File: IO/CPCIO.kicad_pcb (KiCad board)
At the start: 2 copper layers, 99.1 x 52.9 mm, 57 parts, among them IC107 8255A, IC301 LM358, J1 Tape in, J2 Tape out, J3 Motor, J901 Conn_01x07_Male, J902 Conn_01x08_Male, Q101 BC337, Q901 BC337, U1 74LS688

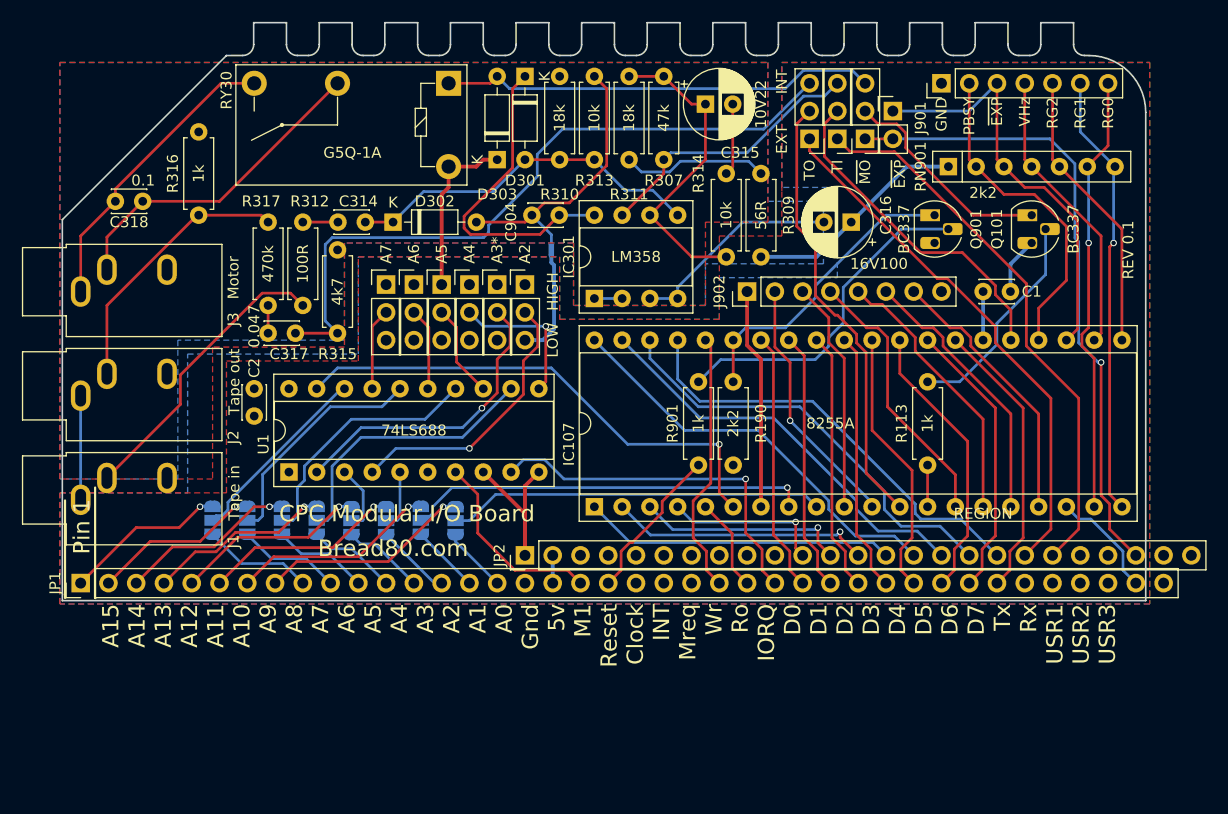
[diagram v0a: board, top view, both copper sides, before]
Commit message: Long overdue update...
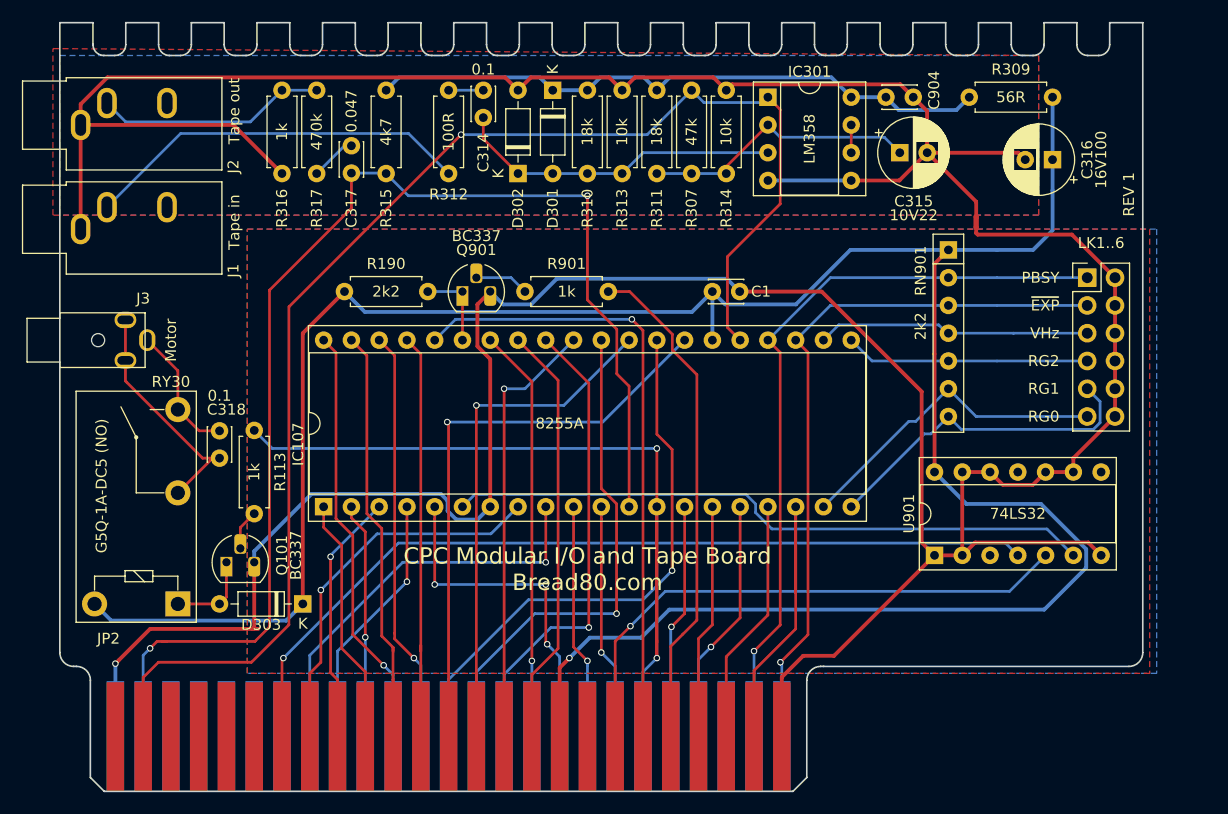
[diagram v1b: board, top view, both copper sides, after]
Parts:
- removed C2: 0.1nF, Capacitor_THT:C_Disc_D3.0mm_W2.0mm_P2.50mm
- removed J901: Conn_01x07_Male, Connector_PinHeader_2.54mm:PinHeader_1x07_P2.54mm_Vertical
- removed J902: Conn_01x08_Male, Connector_PinHeader_2.54mm:PinHeader_1x08_P2.54mm_Vertical
- removed JP10: A14A6, Connector_PinHeader_2.54mm:PinHeader_1x03_P2.54mm_Vertical
- removed JP11, JP17, JP18, JP19: A10A2, Connector_PinHeader_2.54mm:PinHeader_1x03_P2.54mm_Vertical
- removed JP12: A15A7, Connector_PinHeader_2.54mm:PinHeader_1x03_P2.54mm_Vertical
- removed JP13, JP14, JP15, JP16, JP3, JP4, JP7, JP8: Jumper_3_Bridged12, Jumper:SolderJumper-3_P1.3mm_Open_RoundedPad1.0x1.5mm
- removed JP5: A12A4, Connector_PinHeader_2.54mm:PinHeader_1x03_P2.54mm_Vertical
- removed JP6: A13A5, Connector_PinHeader_2.54mm:PinHeader_1x03_P2.54mm_Vertical
- removed JP9: A11A3, Connector_PinHeader_2.54mm:PinHeader_1x03_P2.54mm_Vertical
- removed LK913: Jumper_NO_Small, Connector_PinHeader_2.54mm:PinHeader_1x02_P2.54mm_Vertical
- removed U1: 74LS688, Package_DIP:DIP-20_W7.62mm_Socket
- added LK1..6: Settings, Connector_PinHeader_2.54mm:PinHeader_2x06_P2.54mm_Vertical, F.Cu at (247.7, 123.8)
- added U901: 74LS32, Package_DIP:DIP-14_W7.62mm_Socket, F.Cu at (233.7, 149.2)
- J3: footprint Connector_Audio:Jack_3.5mm_CUI_SJ1-3533NG_Horizontal -> CPCModular:CUI_MJ1_2503A
- JP1: value RC2014Bus -> CPCM_IOSound_EdgeBottom; footprint Connector_PinHeader_2.54mm:PinHeader_1x40_P2.54mm_Vertical -> CPCModular:Edge25_2.54PS; moved to B.Cu
- JP2: value RC2014ExtendedBus -> CPCM_IOSound_EdgeTop; footprint Connector_PinHeader_2.54mm:PinHeader_1x25_P2.54mm_Vertical -> CPCModular:Edge25_2.54PS
- JP20: moved to F.Cu
- RY30: value G5Q-1A -> G5Q-1A-DC5 (NO)
- moved Q101 80.2 mm to (168.9, 149.9), turned to 0 degrees
- moved R113 61.7 mm to (171.4, 137.8), turned to 270 degrees
- moved RY30 53.7 mm to (164.5, 153.7), turned to 90 degrees
- moved D303 44.4 mm to (175.9, 153.7), turned to 180 degrees
- moved Q901 43.7 mm to (190.5, 125.1), turned to 0 degrees
- moved JP2 41.7 mm to (158.8, 167.6)
- moved JP20 38.9 mm to (237.5, 118.7)
- moved R190 38.9 mm to (179.7, 125.1), turned to 0 degrees
- moved C904 31.8 mm to (229.2, 107.3), turned to 0 degrees
- moved R309 30.4 mm to (244.5, 107.3), turned to 180 degrees
- moved J1 24.8 mm to (155.6, 119.4)
- moved J2 24.8 mm to (155.6, 109.9)
- moved C1 24.8 mm to (213.4, 125.1)
- moved IC107 24.8 mm to (177.8, 144.8)
- moved IC301 24.3 mm to (218.4, 107.3), turned to 0 degrees
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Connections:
- C317 pad 2: /IO_SOUND/Tape/CASWRINT -> /IO_SOUND/CASWR
- IC107 pad 12: /IO_SOUND/WR_DATA -> /IO_SOUND/CASWR
- IC107 pad 13: Net-(IC107-Pad13) -> /IO_SOUND/MOTOR
- IC107 pad 25: /IO_SOUND/RD_DATA -> /IO_SOUND/CASRD
- IC107 pad 8: /IO_SOUND/A9A1 -> A9
- IC107 pad 9: /IO_SOUND/A8A0 -> A8
- IC301 pad 1: Net-(IC301-Pad1) -> /IO_SOUND/CASRD
- IC301 pad 2: Net-(IC301-Pad1) -> Net-(C315-Pad1)
- IC301 pad 3: GNDA -> Net-(C314-Pad1)
- IC301 pad 5: Net-(C314-Pad1) -> GNDA
- IC301 pad 6: Net-(C315-Pad1) -> Net-(IC301-Pad6)
- IC301 pad 7: /IO_SOUND/Tape/CASRDINT -> Net-(IC301-Pad6)
- J3 pad S: Net-(C318-Pad1) -> Net-(C318-Pad2)
- J3 pad T: Net-(C318-Pad2) -> Net-(C318-Pad1)
- JP1 pad 1: A15 -> GND
- JP1 pad 10: A6 -> PA2
- JP1 pad 11: A5 -> PA4
- JP1 pad 12: A4 -> PA6
- JP1 pad 13: A3 -> D6
- JP1 pad 14: A2 -> D4
- JP1 pad 15: A1 -> D2
- JP1 pad 16: A0 -> D0
- JP1 pad 17: GND -> /IO_SOUND/~RD
- JP1 pad 18: +5V -> /IO_SOUND/BDIR
- JP1 pad 19: /IO_SOUND/~M1 -> /IO_SOUND/BC1
- JP1 pad 2: A14 -> /IO_SOUND/CASWR
- JP1 pad 20: /IO_SOUND/~RESET -> /IO_SOUND/MOTOR
- JP1 pad 21: Net-(JP1-Pad21) -> PC0
- JP1 pad 22: Net-(JP1-Pad22) -> PC2
- JP1 pad 24: /IO_SOUND/~WR -> /IO_SOUND/PRTBSY
- JP1 pad 25: /IO_SOUND/~RD -> /IO_SOUND/~EXP
- JP1 pad 3: A13 -> Net-(JP1-Pad3)
- JP1 pad 4: A12 -> Net-(JP1-Pad4)
- JP1 pad 5: A11 -> Net-(JP1-Pad5)
- JP1 pad 6: A10 -> Net-(JP1-Pad6)
- JP1 pad 7: A9 -> Net-(JP1-Pad7)
- JP1 pad 9: A7 -> PA0
- JP2 pad 1: GND -> Net-(JP2-Pad1)
- JP2 pad 10: Net-(JP2-Pad10) -> PA3
- JP2 pad 11: PA0 -> PA5
- JP2 pad 12: PA1 -> PA7
- JP2 pad 13: PA2 -> D7
- JP2 pad 14: PA3 -> D5
- JP2 pad 15: PA4 -> D3
- JP2 pad 16: PA5 -> D1
- JP2 pad 17: PA6 -> +5V
- JP2 pad 18: PA7 -> Net-(JP2-Pad18)
- JP2 pad 19: /IO_SOUND/CASWREXT -> /IO_SOUND/~IORQ
- JP2 pad 2: +5V -> /IO_SOUND/CASRD
- JP2 pad 20: /IO_SOUND/CASRDEXT -> /IO_SOUND/~WR
- JP2 pad 21: Net-(JP2-Pad21) -> /IO_SOUND/~RESET
- JP2 pad 22: Net-(JP2-Pad22) -> PC1
- JP2 pad 23: /IO_SOUND/~MOTOREXT -> PC3
- JP2 pad 24: Net-(JP2-Pad24) -> /IO_SOUND/VSYNC
- JP2 pad 25: (no net) -> GND
- JP2 pad 7: Net-(JP2-Pad7) -> A11
- JP2 pad 8: Net-(JP2-Pad8) -> A9
- JP2 pad 9: Net-(JP2-Pad9) -> PA1
- Q101 pad 1: Net-(JP17-Pad2) -> /IO_SOUND/Tape/~MOTORINT
- R113 pad 1: Net-(IC107-Pad13) -> /IO_SOUND/MOTOR
- R307 pad 2: /IO_SOUND/Tape/CASRDINT -> /IO_SOUND/CASRD
- R315 pad 1: /IO_SOUND/Tape/CASWRINT -> /IO_SOUND/CASWR
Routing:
- net +5V: track 43.3 -> 236.1 mm, vias 0 -> 1
- net GND: track 52.7 -> 232.2 mm, vias 0 -> 1
- net /IO_SOUND/CASRD: track 0.00 -> 129.5 mm, vias 0 -> 1
- net /IO_SOUND/CASWR: track 0.00 -> 119.4 mm, vias 0 -> 2
- net GNDA: track 61.6 -> 150.2 mm
- net /IO_SOUND/MOTOR: track 0.00 -> 80.3 mm, vias 0 -> 2
- net /IO_SOUND/Tape/CASWRINT: track 64.4 -> 0.00 mm
- net A11: track 17.5 -> 81.1 mm
- net /IO_SOUND/~MOTOREXT: track 58.4 -> 0.00 mm, vias 1 -> 0
- net /IO_SOUND/CASRDEXT: track 50.6 -> 0.00 mm
- net /IO_SOUND/CASWREXT: track 48.8 -> 0.00 mm
- net /IO_SOUND/PRTBSY: track 29.9 -> 71.1 mm, vias 0 -> 1
- net /IO_SOUND/WR_DATA: track 40.7 -> 0.00 mm
- net /IO_SOUND/A9A1: track 36.9 -> 0.00 mm, vias 1 -> 0
- net /IO_SOUND/~WR: track 24.1 -> 59.2 mm, vias 0 -> 1
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- added copper zone on B.Cu, net +5V
- added copper zone on B.Cu, net +5VA
- added copper zone on F.Cu, net GND
- added copper zone on F.Cu, net GNDA
- removed copper zone on F.Cu, net +5V
- removed copper zone on F.Cu, net +5VA
- removed copper zone on B.Cu, net GND
- removed copper zone on B.Cu, net GNDA
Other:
- board size 99.1 x 52.9 mm -> 99.1 x 70.3 mm
- board text added: "CPC Modular I/O and Tape Board Bread80.com"
- board text added: "CPC Modular: I/O + Tape module Bread80.com © Mike Sutton 2024 @bread80@mstdn.social"
- board text added: "Links: Leave open for defaults. RG0..RG3: Region (manufacturer) VHz: 50Hz/60Hz EXP: Autobook CP/M PBSY: Printer busy"
- board text added: "MOTOR"
- board text added: "Motor"
- board text added: "REV 1"
- board text added: "TAPE IN"
- board text added: "TAPE OUT"
- board text added: "Unless marked otherwise: All caps are 0.1uF All diodes are 1N4148"
- board text removed: "A0"
- board text removed: "A15"
- board text removed: "A15 A14 A13 A12 A11 A10 A9 A8 A7 A6 A5 A4 A3 A2 A1 A0 Gnd 5v M1 Reset Clock INT Mreq Wr Ro IORQ D0 D1 D2 D3 D4 D5 D6 D7 Tx Rx USR1 USR2 USR3"
- board text removed: "A2"
- board text removed: "A3*"
- board text removed: "A4"
- board text removed: "A5"
- board text removed: "A6"
- board text removed: "A7"
- board text removed: "AY BUS"
- board text removed: "Bread80.com"
- board text removed: "Bread80.com © Mike Sutton 2022 @bread80@mstdn.social"
- board text removed: "CPC Modular I/O Board"
- board text removed: "CPC Modular for RC2014 backplane I/O module"
- board text removed: "EXT"
- board text removed: "GND"
- board text removed: "HIGH"
- board text removed: "I/O address select"
- board text removed: "INT"
- board text removed: "Jumpers to internal or backplane"
- board text removed: "LOW"
- board text removed: "Mezzanine to sound board"
- board text removed: "Pin 1"
- board text removed: "REGION"
- board text removed: "REV 0.1"
- board text removed: "Select I/O address bus high or low byte"
- board text removed: "TI"
- board text removed: "TO"
- board text removed: "USR3/6=VSYNC/~MOTOR"
- board text removed: "~MO"
